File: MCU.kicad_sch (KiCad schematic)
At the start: 15 parts, among them J3 Conn_02x03_Odd_Even, U1 HDC2080, U3 ESP32-C6-MINI-1

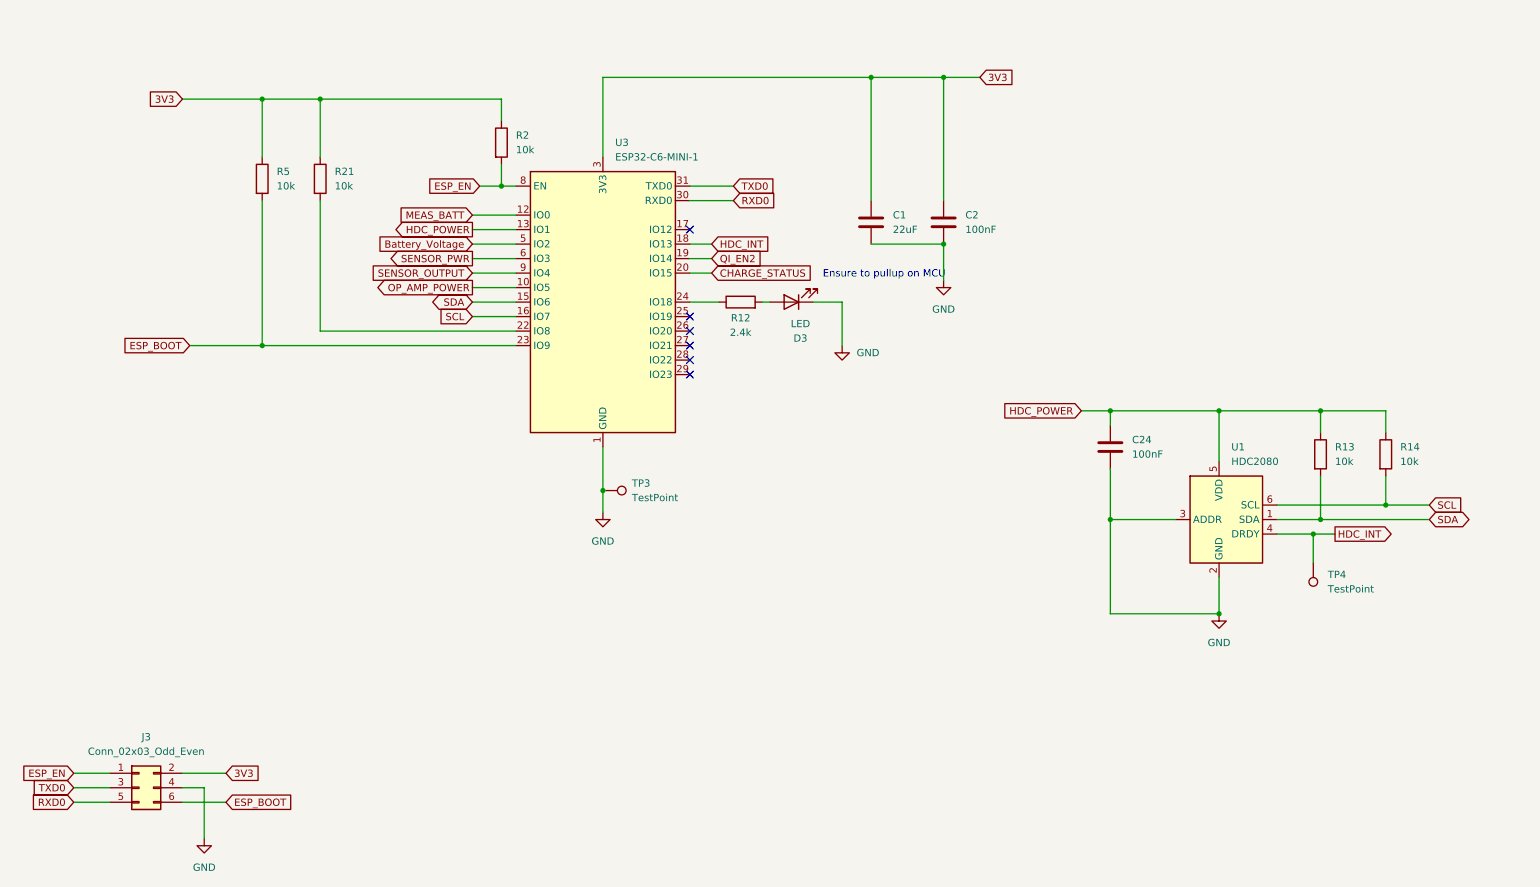
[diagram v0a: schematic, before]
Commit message: finished board layout for AD revision
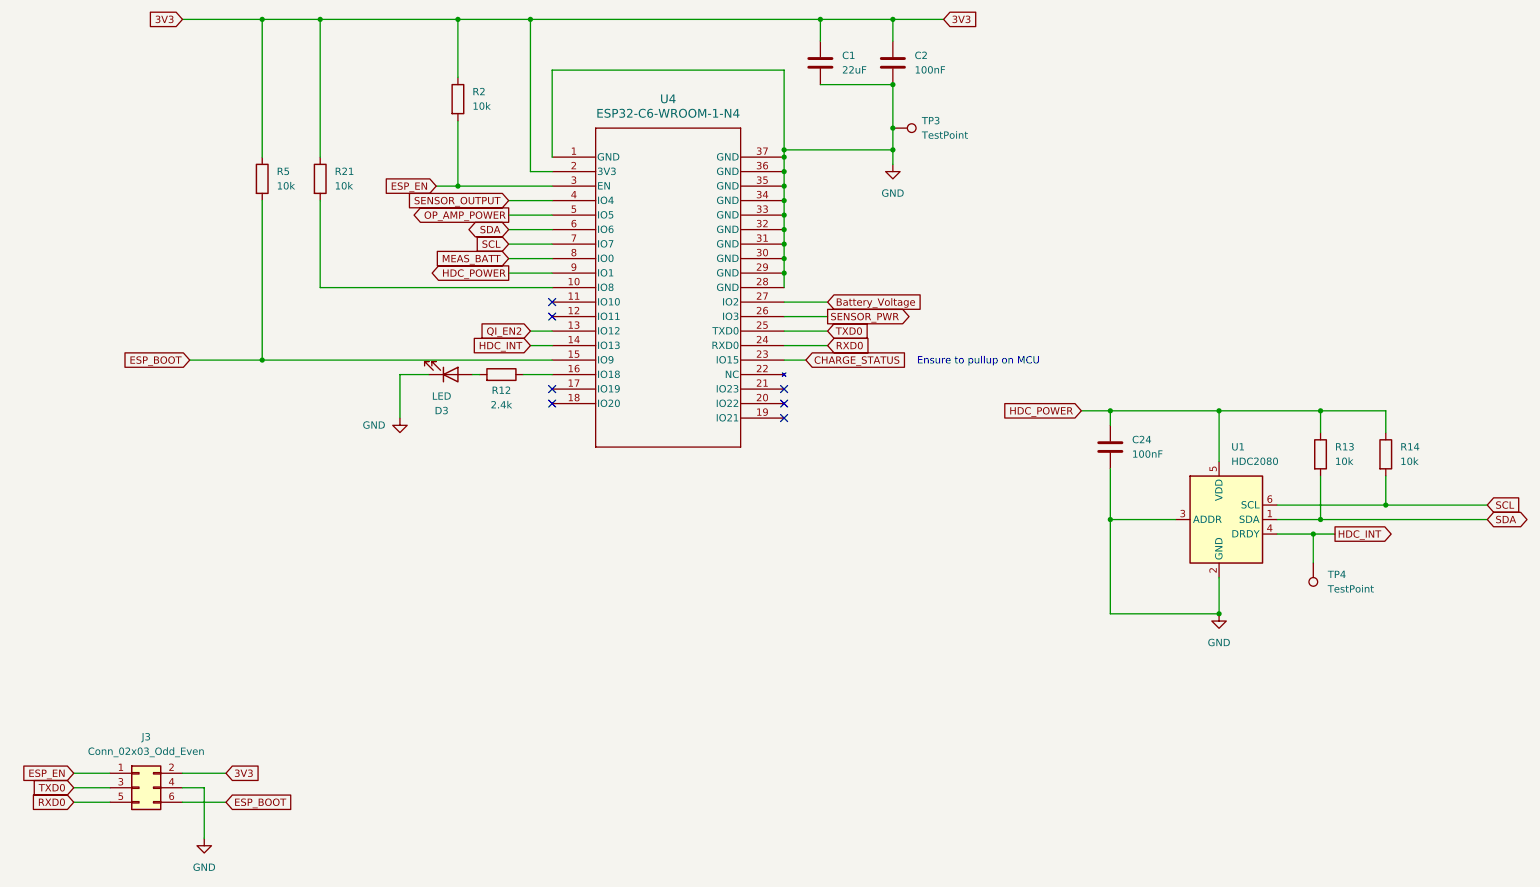
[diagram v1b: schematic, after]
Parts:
- removed U3: ESP32-C6-MINI-1, RF_Module:ESP32-C6-MINI-1, symbol RF_Module:ESP32-C6-MINI-1
- added U4: ESP32-C6-WROOM-1-N4, Hydro_footprints:MOD28_ESP32-C6-WROOM-1_EXP, symbol Hydro_symbols:ESP32-C6-WROOM-1-N4
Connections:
- net 3V3: now also U4.2 (3V3)
- net Battery_Voltage: now also U4.27 (IO2)
- net CHARGE_STATUS: now also U4.23 (IO15)
- net ESP_BOOT: now also U4.15 (IO9)
- net ESP_EN: now also U4.3 (EN)
- net GND: now also U4.1 (GND), U4.28 (GND), U4.29 (GND), U4.30 (GND), U4.31 (GND), U4.32 (GND), U4.33 (GND), U4.34 (GND), U4.35 (GND), U4.36 (GND), U4.37 (GND)
- net HDC_INT: now also U4.14 (IO13)
- net HDC_POWER: now also U4.9 (IO1)
- net MEAS_BATT: now also U4.8 (IO0)
- net OP_AMP_POWER: now also U4.5 (IO5)
- net QI_EN2: now also U4.13 (IO12)
- net RXD0: now also U4.24 (RXD0)
- net SCL: now also U4.7 (IO7)
- net SDA: now also U4.6 (IO6)
- net SENSOR_OUTPUT: now also U4.4 (IO4)
- net SENSOR_PWR: now also U4.26 (IO3)
- net TXD0: now also U4.25 (TXD0)
- net at R12.1: now also U4.16 (IO18)
- net at R21.2: now also U4.10 (IO8)
- no-connect marks 6 -> 7
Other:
- moved on the sheet: C1, C2, D3, R12, R2
